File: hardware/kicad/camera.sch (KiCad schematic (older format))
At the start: 69 parts

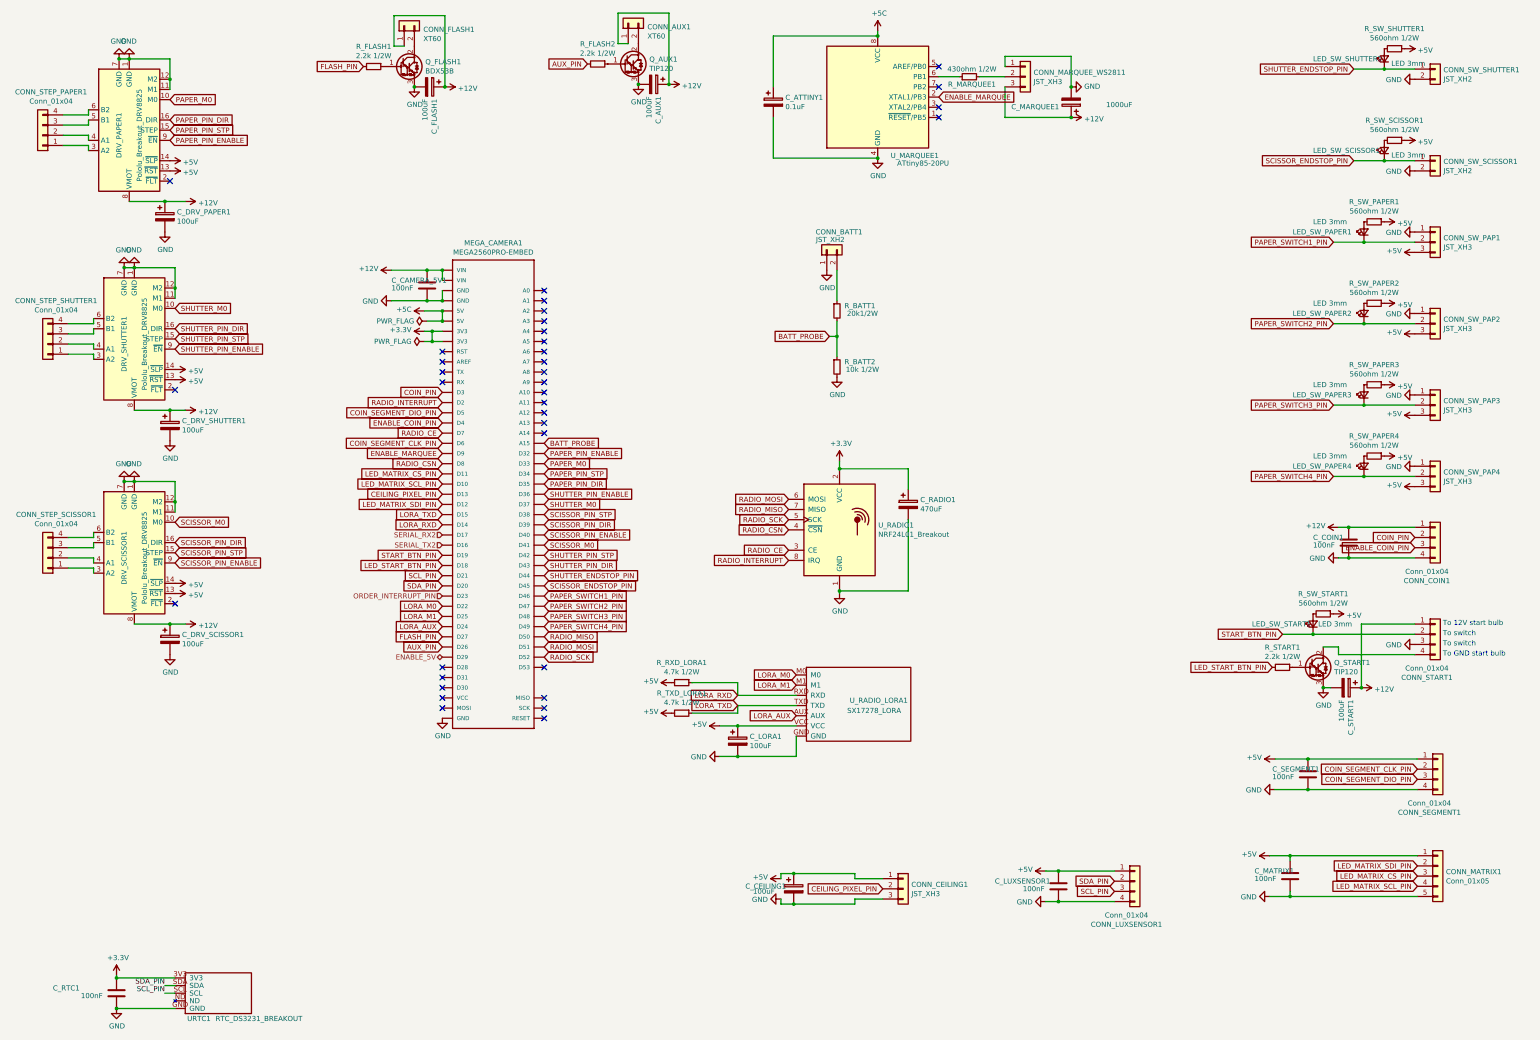
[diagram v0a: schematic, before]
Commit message: update, gilou dans la place
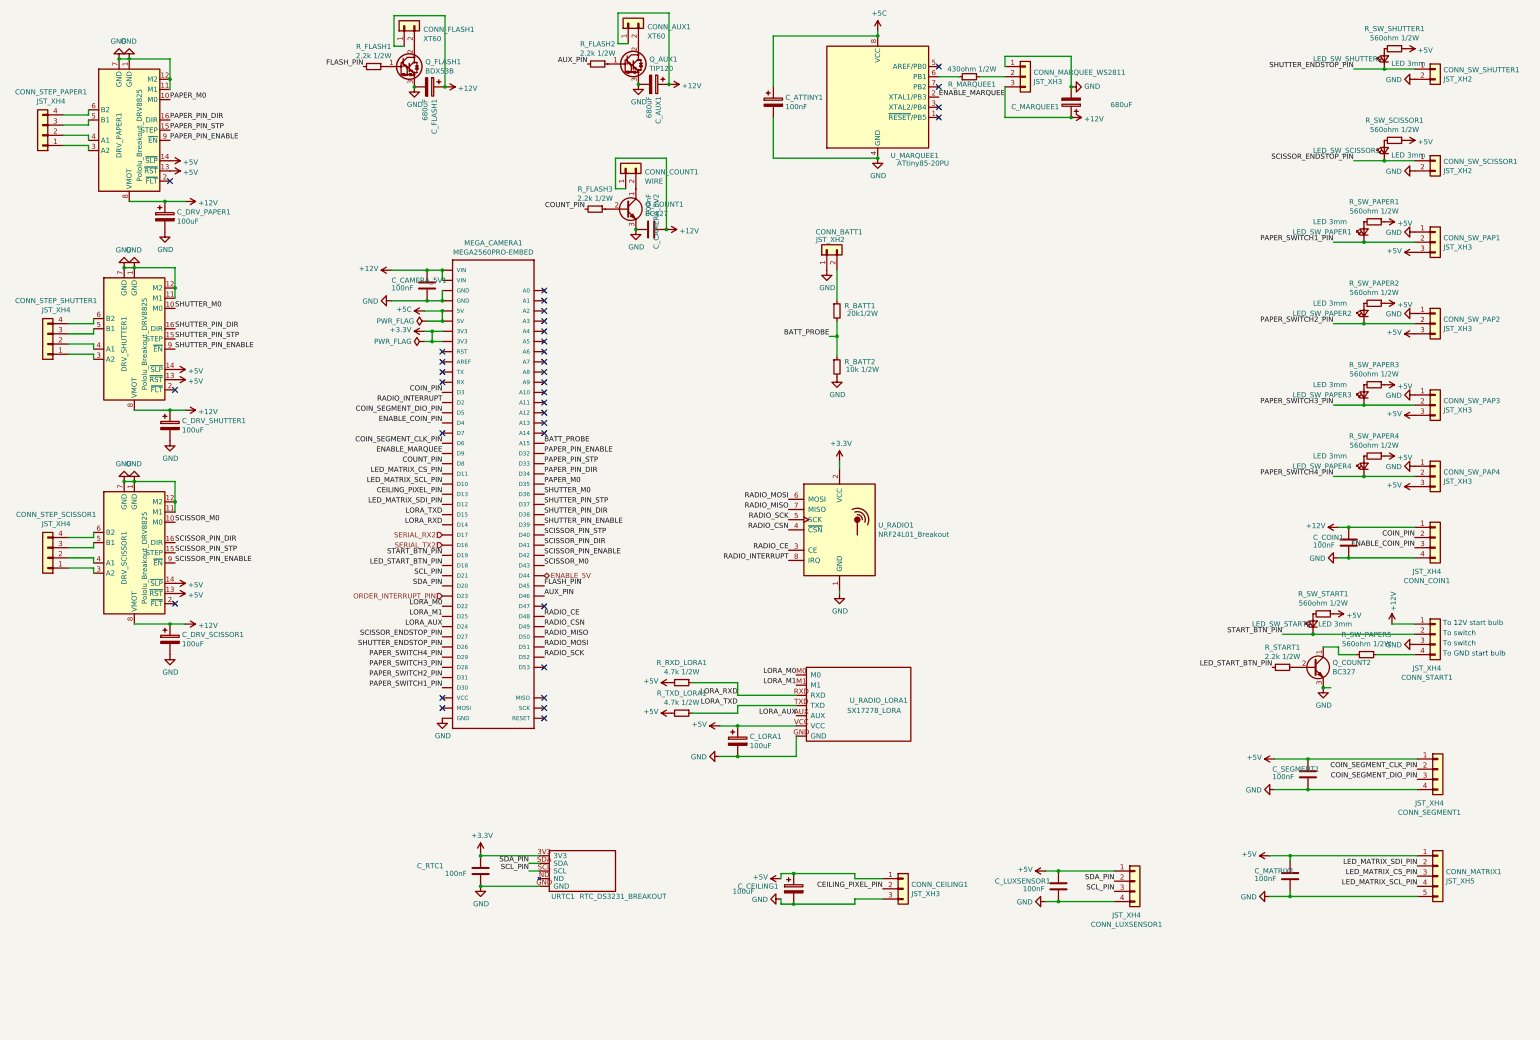
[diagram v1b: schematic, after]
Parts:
- removed C_RADIO1: 470uF, Capacitor_THT:CP_Radial_D10.0mm_P5.00mm, symbol 1nofilterbooth:CP-Device
- removed C_START1: 100uF, Capacitor_THT:CP_Radial_D10.0mm_P5.00mm, symbol 1nofilterbooth:CP-Device
- removed Q_START1: TIP120, Package_TO_SOT_THT:TO-220-3_Vertical, symbol 1nofilterbooth:TIP120-Transistor_BJT
- added CONN_COUNT1: WIRE, Connector_PinHeader_2.54mm:PinHeader_1x02_P2.54mm_Vertical, symbol 1nofilterbooth:Conn_01x02-Connector_Generic
- added C_CAMERA_5V2: 100nF, Capacitor_THT:C_Rect_L7.2mm_W2.5mm_P5.00mm_FKS2_FKP2_MKS2_MKP2, symbol 1nofilterbooth:C-Device
- added Q_COUNT1, Q_COUNT2: BC327, Package_TO_SOT_THT:TO-92L_HandSolder, symbol Device:Q_NPN_CBE
- added R_FLASH3: 2.2k 1/2W, Resistor_THT:R_Axial_DIN0207_L6.3mm_D2.5mm_P10.16mm_Horizontal, symbol 1nofilterbooth:R_Small-Device
- added R_SW_PAPER5: 560ohm 1/2W, Resistor_THT:R_Axial_DIN0207_L6.3mm_D2.5mm_P10.16mm_Horizontal, symbol 1nofilterbooth:R_Small-Device
- CONN_BATT1, CONN_SW_SCISSOR1, CONN_SW_SHUTTER1: footprint Connector_JST:JST_XH_S2B-XH-A_1x02_P2.50mm_Horizontal -> Connector_JST:JST_XH_S2B-XH-A-1_1x02_P2.50mm_Horizontal
- CONN_CEILING1, CONN_MARQUEE_WS2811, CONN_SW_PAP1, CONN_SW_PAP2, CONN_SW_PAP3, CONN_SW_PAP4: footprint Connector_JST:JST_XH_S3B-XH-A_1x03_P2.50mm_Horizontal -> Connector_JST:JST_XH_S3B-XH-A-1_1x03_P2.50mm_Horizontal
- CONN_COIN1, CONN_LUXSENSOR1, CONN_SEGMENT1, CONN_START1, CONN_STEP_PAPER1, CONN_STEP_SCISSOR1, CONN_STEP_SHUTTER1: value Conn_01x04 -> JST_XH4; footprint Connector_JST:JST_XH_S4B-XH-A_1x04_P2.50mm_Horizontal -> Connector_JST:JST_XH_S4B-XH-A-1_1x04_P2.50mm_Horizontal
- CONN_MATRIX1: value Conn_01x05 -> JST_XH5; footprint Connector_JST:JST_XH_S5B-XH-A_1x05_P2.50mm_Horizontal -> Connector_JST:JST_XH_S5B-XH-A-1_1x05_P2.50mm_Horizontal
- C_ATTINY1: value 0.1uF -> 100nF
- C_AUX1, C_FLASH1: value 100uF -> 680uF; footprint Capacitor_THT:CP_Radial_D10.0mm_P5.00mm -> Capacitor_THT:CP_Radial_D8.0mm_P3.50mm
- C_CEILING1, C_DRV_PAPER1, C_DRV_SCISSOR1, C_DRV_SHUTTER1, C_LORA1: footprint Capacitor_THT:CP_Radial_D10.0mm_P5.00mm -> Capacitor_THT:CP_Radial_D6.3mm_P2.50mm
- C_MARQUEE1: value 1000uF -> 680uF; footprint Capacitor_THT:CP_Radial_D10.0mm_P5.00mm -> Capacitor_THT:CP_Radial_D8.0mm_P3.50mm
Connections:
- net +12V: now also CONN_COUNT1.1 (Pin_1), C_CAMERA_5V2.1
- net AUX_PIN: now also MEGA_CAMERA1.D46; no longer MEGA_CAMERA1.D26
- net ENABLE_5V: now also MEGA_CAMERA1.D44; no longer MEGA_CAMERA1.D29
- net FLASH_PIN: now also MEGA_CAMERA1.D45; no longer MEGA_CAMERA1.D27
- net GND: now also C_CAMERA_5V2.2, Q_COUNT1.3 (E), Q_COUNT2.3 (E)
- net PAPER_M0: now also MEGA_CAMERA1.D35; no longer MEGA_CAMERA1.D33
- net PAPER_PIN_DIR: now also MEGA_CAMERA1.D34; no longer MEGA_CAMERA1.D35
- net PAPER_PIN_STP: now also MEGA_CAMERA1.D33; no longer MEGA_CAMERA1.D34
- net PAPER_SWITCH1_PIN: now also MEGA_CAMERA1.D30; no longer MEGA_CAMERA1.D46
- net PAPER_SWITCH2_PIN: now also MEGA_CAMERA1.D31; no longer MEGA_CAMERA1.D47
- net PAPER_SWITCH3_PIN: now also MEGA_CAMERA1.D28; no longer MEGA_CAMERA1.D48
- net PAPER_SWITCH4_PIN: now also MEGA_CAMERA1.D29; no longer MEGA_CAMERA1.D49
- net RADIO_CE: now also MEGA_CAMERA1.D48; no longer MEGA_CAMERA1.D7
- net RADIO_CSN: now also MEGA_CAMERA1.D49; no longer MEGA_CAMERA1.D8
- net SCISSOR_ENDSTOP_PIN: now also MEGA_CAMERA1.D27; no longer MEGA_CAMERA1.D45
- net SCISSOR_M0: now also MEGA_CAMERA1.D43; no longer MEGA_CAMERA1.D41
- net SCISSOR_PIN_DIR: now also MEGA_CAMERA1.D41; no longer MEGA_CAMERA1.D39
- net SCISSOR_PIN_ENABLE: now also MEGA_CAMERA1.D42; no longer MEGA_CAMERA1.D40
- net SCISSOR_PIN_STP: now also MEGA_CAMERA1.D40; no longer MEGA_CAMERA1.D38
- net SHUTTER_ENDSTOP_PIN: now also MEGA_CAMERA1.D26; no longer MEGA_CAMERA1.D44
- net SHUTTER_M0: now also MEGA_CAMERA1.D36; no longer MEGA_CAMERA1.D37
- net SHUTTER_PIN_DIR: now also MEGA_CAMERA1.D38; no longer MEGA_CAMERA1.D43
- net SHUTTER_PIN_ENABLE: now also MEGA_CAMERA1.D39; no longer MEGA_CAMERA1.D36
- net SHUTTER_PIN_STP: now also MEGA_CAMERA1.D37; no longer MEGA_CAMERA1.D42
- net at CONN_START1.4 (Pin_4): now also R_SW_PAPER5.1
- net at R_START1.1: now also Q_COUNT2.2 (B)
- new net: CONN_COUNT1.2 (Pin_2), Q_COUNT1.1 (C)
- new net: Q_COUNT1.2 (B), R_FLASH3.1
- new net: Q_COUNT2.1 (C), R_SW_PAPER5.2
- new net COUNT_PIN: MEGA_CAMERA1.D8, R_FLASH3.2
- no-connect marks 35 -> 34
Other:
- moved on the sheet: C_RTC1, URTC1
